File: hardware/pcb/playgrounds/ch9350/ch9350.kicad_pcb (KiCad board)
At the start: 2 copper layers, 50.8 x 106.7 mm, 0 parts

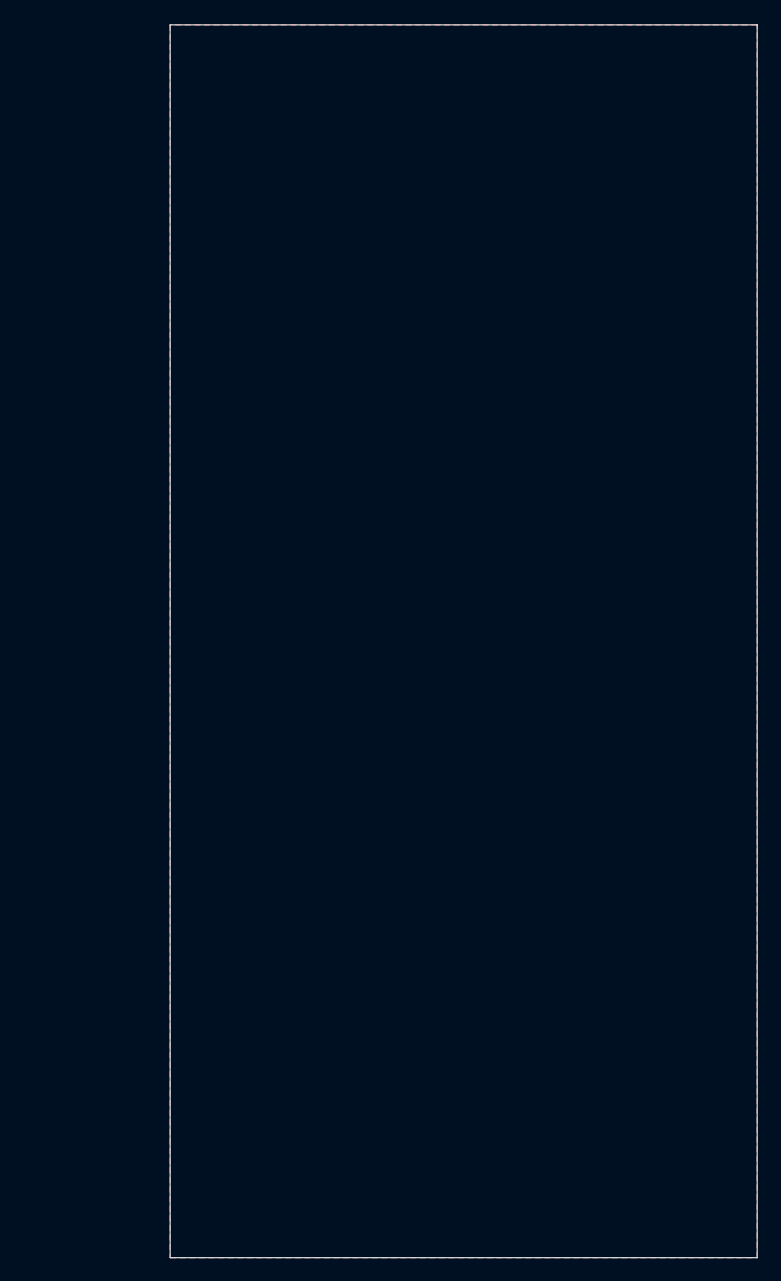
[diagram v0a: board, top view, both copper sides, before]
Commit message: ch9350 devboard layout 3?
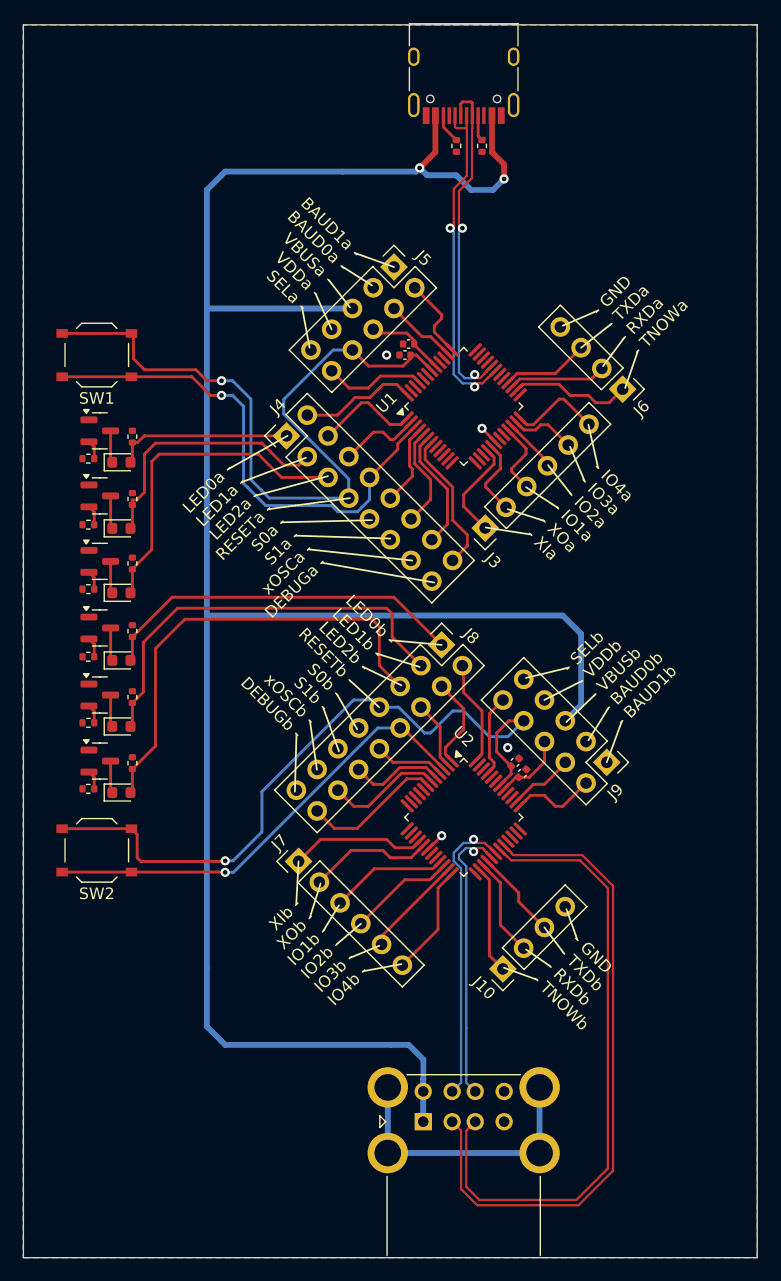
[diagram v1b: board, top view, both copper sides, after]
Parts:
- added C1: 4u7F, Capacitor_SMD:C_0402_1005Metric, F.Cu at (147.3, 79.4)
- added C2: 100nF, Capacitor_SMD:C_0402_1005Metric, F.Cu at (147.6, 78.4)
- added C3: 4u7F, Capacitor_SMD:C_0402_1005Metric, F.Cu at (156.8, 114.6)
- added C4: 100nF, Capacitor_SMD:C_0402_1005Metric, F.Cu at (157.5, 115.6)
- added D1: 19-213/Y2C-CQ2R2L/3T(CY), LED_SMD:LED_0603_1608Metric, F.Cu at (122.8, 88.7)
- added D2: 19-213/Y2C-CQ2R2L/3T(CY), LED_SMD:LED_0603_1608Metric, F.Cu at (122.8, 94.4)
- added D3: 19-213/Y2C-CQ2R2L/3T(CY), LED_SMD:LED_0603_1608Metric, F.Cu at (122.8, 100.0)
- added D4: 19-213/Y2C-CQ2R2L/3T(CY), LED_SMD:LED_0603_1608Metric, F.Cu at (122.8, 105.8)
- added D5: 19-213/Y2C-CQ2R2L/3T(CY), LED_SMD:LED_0603_1608Metric, F.Cu at (122.8, 111.5)
- added D6: 19-213/Y2C-CQ2R2L/3T(CY), LED_SMD:LED_0603_1608Metric, F.Cu at (122.8, 117.2)
- added J1: TYPE-C-31-M-12, Connector_USB:USB_C_Receptacle_HRO_TYPE-C-31-M-12, F.Cu at (152.4, 54.6)
- added J10: Conn_01x04, Connector_PinHeader_2.54mm:PinHeader_1x04_P2.54mm_Vertical, F.Cu at (155.8, 132.5)
- added J2: USB-U267-BWS, Connector_USB:USB_A_CUI_UJ2-ADH-TH_Horizontal_Stacked, F.Cu at (148.9, 145.7)
- added J3: Conn_01x06, Connector_PinHeader_2.54mm:PinHeader_1x06_P2.54mm_Vertical, F.Cu at (154.3, 94.3)
- added J4: Conn_02x08, Connector_PinHeader_2.54mm:PinHeader_2x08_P2.54mm_Vertical, F.Cu at (137.1, 86.4)
- added J5: Conn_02x05, Connector_PinHeader_2.54mm:PinHeader_2x05_P2.54mm_Vertical, F.Cu at (146.4, 71.8)
- added J6: Conn_01x04, Connector_PinHeader_2.54mm:PinHeader_1x04_P2.54mm_Vertical, F.Cu at (166.2, 82.3)
- added J7: Conn_01x06, Connector_PinHeader_2.54mm:PinHeader_1x06_P2.54mm_Vertical, F.Cu at (138.1, 123.2)
- added J8: Conn_02x08, Connector_PinHeader_2.54mm:PinHeader_2x08_P2.54mm_Vertical, F.Cu at (150.5, 104.5)
- added J9: Conn_02x05, Connector_PinHeader_2.54mm:PinHeader_2x05_P2.54mm_Vertical, F.Cu at (164.8, 114.6)
- added Q1: MMBT2222A, Package_TO_SOT_SMD:SOT-23, F.Cu at (120.9, 85.9)
- added Q2: MMBT2222A, Package_TO_SOT_SMD:SOT-23, F.Cu at (120.9, 91.6)
- added Q3: MMBT2222A, Package_TO_SOT_SMD:SOT-23, F.Cu at (120.9, 97.2)
- added Q4: MMBT2222A, Package_TO_SOT_SMD:SOT-23, F.Cu at (120.9, 103.0)
- added Q5: MMBT2222A, Package_TO_SOT_SMD:SOT-23, F.Cu at (120.9, 108.8)
- added Q6: MMBT2222A, Package_TO_SOT_SMD:SOT-23, F.Cu at (120.9, 114.5)
- added R1: 5K1, Resistor_SMD:R_0402_1005Metric, F.Cu at (154.0, 61.3)
- added R10: 6K2, Resistor_SMD:R_0402_1005Metric, F.Cu at (119.9, 105.5)
- added R11: 1K, Resistor_SMD:R_0402_1005Metric, F.Cu at (123.7, 109.0)
- added R12: 6K2, Resistor_SMD:R_0402_1005Metric, F.Cu at (119.9, 111.2)
- added R13: 1K, Resistor_SMD:R_0402_1005Metric, F.Cu at (123.7, 114.7)
- added R14: 6K2, Resistor_SMD:R_0402_1005Metric, F.Cu at (119.9, 116.9)
- added R2: 5K1, Resistor_SMD:R_0402_1005Metric, F.Cu at (151.8, 61.3)
- added R3: 1K, Resistor_SMD:R_0402_1005Metric, F.Cu at (123.7, 86.4)
- added R4: 6K2, Resistor_SMD:R_0402_1005Metric, F.Cu at (119.9, 88.3)
- added R5: 1K, Resistor_SMD:R_0402_1005Metric, F.Cu at (123.7, 91.8)
- added R6: 6K2, Resistor_SMD:R_0402_1005Metric, F.Cu at (119.9, 94.1)
- added R7: 1K, Resistor_SMD:R_0402_1005Metric, F.Cu at (123.7, 97.4)
- added R8: 6K2, Resistor_SMD:R_0402_1005Metric, F.Cu at (119.9, 99.6)
- added R9: 1K, Resistor_SMD:R_0402_1005Metric, F.Cu at (123.7, 103.3)
- added SW1: TS-1187A-B-A-B, Button_Switch_SMD:SW_Push_1P1T_XKB_TS-1187A, F.Cu at (120.7, 79.4)
- added SW2: TS-1187A-B-A-B, Button_Switch_SMD:SW_Push_1P1T_XKB_TS-1187A, F.Cu at (120.7, 122.2)
- added U1: CH9350L, Package_QFP:LQFP-48_7x7mm_P0.5mm, F.Cu at (152.4, 83.8)
- added U2: CH9350L, Package_QFP:LQFP-48_7x7mm_P0.5mm, F.Cu at (152.4, 119.4)
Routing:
- net /VBUS: track 0.00 -> 190.2 mm, vias 0 -> 2
- net /VDDa: track 0.00 -> 63.1 mm, vias 0 -> 1
- net /VDDb: track 0.00 -> 61.8 mm, vias 0 -> 1
- net /D1-: track 0.00 -> 56.7 mm
- net /D1+: track 0.00 -> 54.8 mm
- net /RESETa: track 0.00 -> 43.8 mm, vias 0 -> 1
- net /JLED2b: track 0.00 -> 40.0 mm
- net /RESETb: track 0.00 -> 39.6 mm, vias 0 -> 1
- net /JLED1b: track 0.00 -> 36.2 mm
- net /JLED0b: track 0.00 -> 32.1 mm
- net /D-: track 0.00 -> 29.9 mm, vias 0 -> 2
- net /D+: track 0.00 -> 29.8 mm, vias 0 -> 2
- net /JLED2a: track 0.00 -> 28.5 mm
- net /D2-: track 0.00 -> 25.8 mm, vias 0 -> 1
- net /D2+: track 0.00 -> 24.7 mm, vias 0 -> 1
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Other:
- board size 50.8 x 106.7 mm -> 63.5 x 106.7 mm
- board text added: "- GND - TXDa - RXDa - TNOWa"
- board text added: "- GND - TXDb - RXDb - TNOWb"
- board text added: "- IO4a - IO3a - IO2a - IO1a - XOa - XIa"
- board text added: "- SELb - VDDb - VBUSb - BAUD0b - BAUD1b"
- board text added: "BAUD1a - BAUD0a - VBUSa - VDDa - SELa -"
- board text added: "LED0a - LED1a - LED2a - RESETa - S0a - S1a - xOSCa - DEBUGa -"
- board text added: "LED0b - LED1b - LED2b - RESETb - S0b - S1b - xOSCb - DEBUGb -"
- board text added: "XIb - XOb - IO1b - IO2b - IO3b - IO4b -"
